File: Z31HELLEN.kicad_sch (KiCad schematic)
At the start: 2 parts, among them CON1 Z32 2024, CON2 Z32 2024

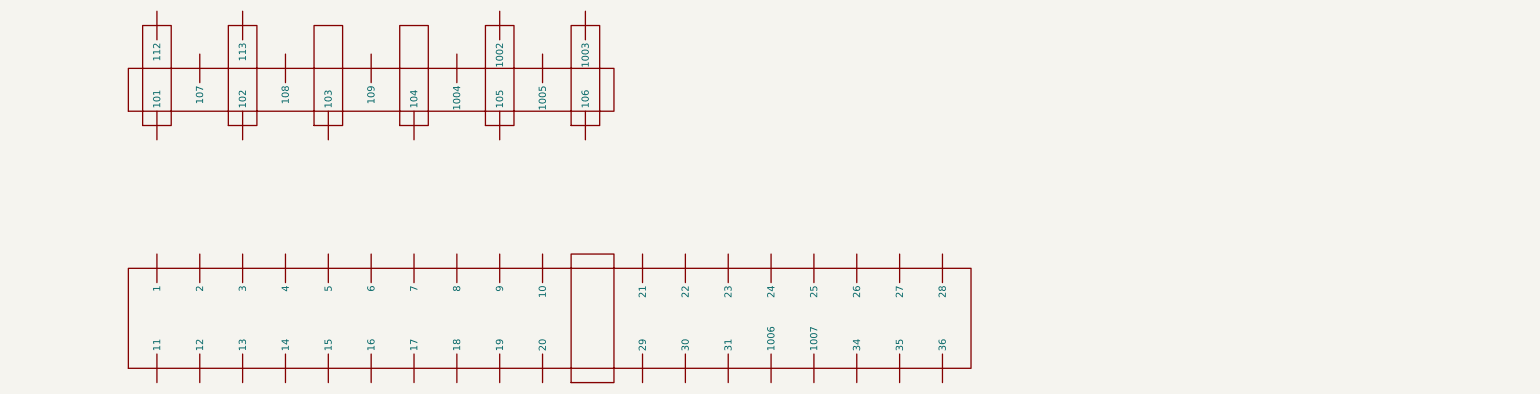
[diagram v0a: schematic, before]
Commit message: Add files via upload
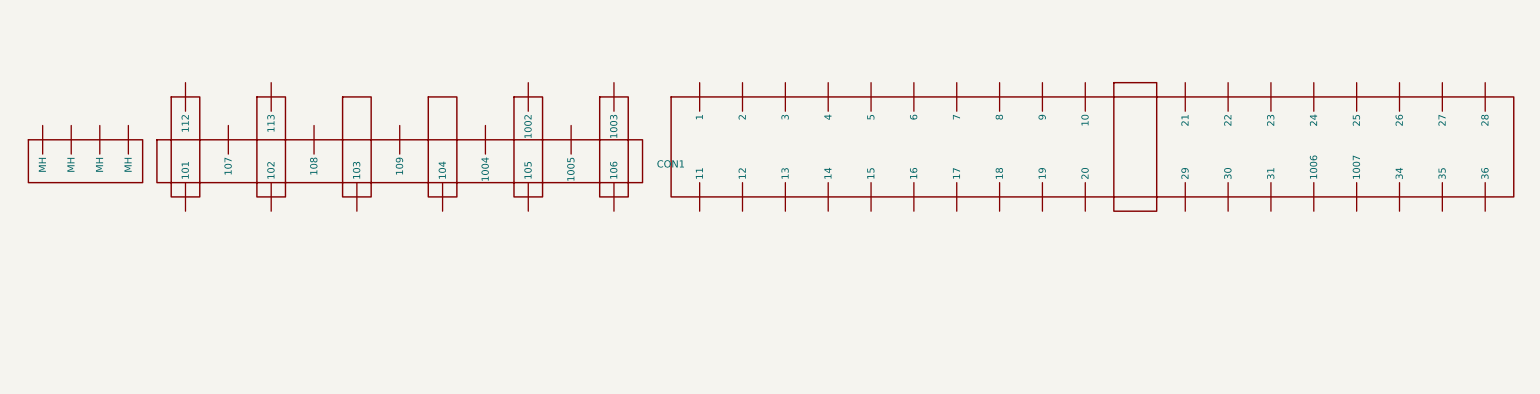
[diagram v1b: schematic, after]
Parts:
- removed CON1: Z32 2024, Main Conne-easyedapro:Z32 2024, symbol z31 15p:Z32 2024
- removed CON2: Z32 2024, Main Conne-easyedapro:Z32 2024, symbol 172023-1:Z32 2024
- added CON1: Z32 2024, symbol Z31HELLEN-altium-import:root_0_Z32 2024
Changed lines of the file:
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@@
 	(generator "eeschema")
 	(generator_version "8.0")
-	(paper "A4")
+	(paper "User" 274.32 99.06)
 	(symbol
-		(lib_id "z31 15p:Z32 2024")
-		(at 111.76 39.37 0)
+		(lib_id "Z31HELLEN-altium-import:root_0_Z32 2024")
+		(at 116.84 52.07 0)
 		(unit 1)
 		(exclude_from_sim no)
@@
 		(on_board yes)
 		(dnp no)
-		(fields_autoplaced yes)
 		(property "Reference" "CON1"
-			(at 265.43 24.13 0)
-			(effects
-				(font
-					(size 1.27 1.27)
-				)
-				(justify left bottom)
-				(hide yes)
+			(at 116.84 52.07 0)
+			(effects
+				(font
+					(size 1.27 1.27)
+				)
+				(justify left bottom)
 			)
 		)
 		(property "Value" "Z32 2024"
-			(at 265.43 26.162 0)
-			(effects
-				(font
-					(size 1.27 1.27)
-				)
-				(justify left bottom)
-				(hide yes)
-			)
-		)
-		(property "Footprint" "Main Conne-easyedapro:Z32 2024"
-			(at 111.76 39.37 0)
+			(at 116.84 52.07 0)
+			(effects
+				(font
+					(size 1.27 1.27)
+				)
+				(justify left bottom)
+				(hide yes)
+			)
+		)
+		(property "Footprint" ""
+			(at 116.84 52.07 0)
 			(effects
 				(font
@@
 		)
 		(property "Datasheet" ""
-			(at 111.76 39.37 0)
+			(at 116.84 52.07 0)
 			(effects
 				(font
@@
 		)
 		(property "Description" ""
-			(at 111.76 39.37 0)
-			(effects
-				(font
-					(size 1.27 1.27)
-				)
-				(hide yes)
-			)
+			(at 116.84 52.07 0)
+			(effects
+				(font
+					(size 1.27 1.27)
+				)
+				(hide yes)
+			)
+		)
+		(property "NAME" ""
+			(at 116.84 52.07 0)
+			(effects
+				(font
+					(size 1.27 1.27)
+				)
+				(justify left bottom)
+				(hide yes)
+			)
+		)
+		(property "SYMBOL" "Z32 2024"
+			(at 116.84 52.07 0)
+			(effects
+				(font
+					(size 1.27 1.27)
+				)
+				(justify left bottom)
+				(hide yes)
+			)
+		)
+		(property "DEVICE" "Z32 2024"
+			(at 116.84 52.07 0)
+			(effects
+				(font
+					(size 1.27 1.27)
+				)
+				(justify left bottom)
+				(hide yes)
+			)
+		)
+		(property "ADD INTO BOM" "yes"
+			(at 116.84 52.07 0)
+			(effects
+				(font
+					(size 1.27 1.27)
+				)
+				(justify left bottom)
+				(hide yes)
+			)
+		)
+		(property "CONVERT TO PCB" "yes"
+			(at 116.84 52.07 0)
+			(effects
+				(font
+					(size 1.27 1.27)
+				)
+				(justify left bottom)
+				(hide yes)
+			)
+		)
+		(property "MANUFACTURER" ""
+			(at 116.84 52.07 0)
+			(effects
+				(font
+					(size 1.27 1.27)
+				)
+				(justify left bottom)
+				(hide yes)
+			)
+		)
+		(property "MANUFACTURER PART" ""
+			(at 116.84 52.07 0)
+			(effects
+				(font
+					(size 1.27 1.27)
+				)
+				(justify left bottom)
+				(hide yes)
+			)
+		)
+		(property "SUPPLIER" ""
+			(at 116.84 52.07 0)
+			(effects
+				(font
+					(size 1.27 1.27)
+				)
+				(justify left bottom)
+				(hide yes)
+			)
+		)
+		(property "SUPPLIER PART" ""
+			(at 116.84 52.07 0)
+			(effects
+				(font
+					(size 1.27 1.27)
+				)
+				(justify left bottom)
+				(hide yes)
+			)
+		)
+		(property "_" "3"
+			(at 116.84 52.07 0)
+			(effects
+				(font
+					(size 1.27 1.27)
+				)
+				(justify left bottom)
+				(hide yes)
+			)
+		)
+		(property "DESCRIPTION" ""
+			(at 116.84 52.07 0)
+			(effects
+				(font
+					(size 1.27 1.27)
+				)
+				(justify left bottom)
+				(hide yes)
+			)
+		)
+		(pin "1008"
+		)
+		(pin "104"
+		)
+		(pin "106"
+		)
+		(pin "105"
+		)
+		(pin "103"
+		)
+		(pin "1007"
+		)
+		(pin "29"
+		)
+		(pin "30"
+		)
+		(pin "35"
+		)
+		(pin "28"
+		)
+		(pin "31"
+		)
+		(pin "27"
+		)
+		(pin "26"
+		)
+		(pin "3"
+		)
+		(pin "36"
+		)
+		(pin "1006"
+		)
+		(pin "107"
+		)
+		(pin "1005"
+		)
+		(pin "108"
+		)
+		(pin "1002"
+		)
+		(pin "1004"
+		)
+		(pin "112"
+		)
+		(pin "109"
+		)
+		(pin "1003"
+		)
+		(pin "101"
+		)
+		(pin "113"
 		)
 		(pin "102"
 		)
-		(pin "103"
-		)
-		(pin "1003"
-		)
-		(pin "101"
-		)
-		(pin "109"
-		)
-		(pin "105"
-		)
-		(pin "108"
-		)
-		(pin "112"
-		)
-		(pin "1004"
-		)
-		(pin "113"
-		)
-		(pin "107"
-		)
-		(pin "106"
-		)
-		(pin "1002"
-		)
-		(pin "104"
-		)
-		(pin "1005"
+		(pin "10010"
+		)
+		(pin "1009"
+		)
+		(pin "10011"
+		)
+		(pin "25"
+		)
+		(pin "16"
+		)
+		(pin "15"
+		)
+		(pin "23"
+		)
+		(pin "22"
+		)
+		(pin "20"
+		)
+		(pin "18"
+		)
+		(pin "17"
+		)
+		(pin "24"
+		)
+		(pin "21"
+		)
+		(pin "19"
+		)
+		(pin "34"
+		)
+		(pin "2"
+		)
+		(pin "1"
+		)
+		(pin "14"
+		)
+		(pin "12"
+		)
+		(pin "11"
+		)
+		(pin "9"
+		)
+		(pin "5"
+		)
+		(pin "10"
+		)
+		(pin "7"
+		)
+		(pin "6"
+		)
+		(pin "4"
+		)
+		(pin "13"
+		)
+		(pin "8"
 		)
 		(instances
 			(project ""
-				(path "/8bd93ac5-a5f9-4744-8cea-27f2f6693e74"
+				(path "/b506e640-3a9c-47d7-91fd-18e11bf19b9e"
 					(reference "CON1")
-					(unit 1)
-				)
-			)
-		)
-	)
-	(symbol
-		(lib_id "172023-1:Z32 2024")
-		(at 20.32 82.55 0)
-		(unit 1)
-		(exclude_from_sim no)
-		(in_bom yes)
-		(on_board yes)
-		(dnp no)
-		(fields_autoplaced yes)
-		(property "Reference" "CON2"
-			(at 173.99 67.31 0)
-			(effects
-				(font
-					(size 1.27 1.27)
-				)
-				(justify left bottom)
-				(hide yes)
-			)
-		)
-		(property "Value" "Z32 2024"
-			(at 173.99 69.342 0)
-			(effects
-				(font
-					(size 1.27 1.27)
-				)
-				(justify left bottom)
-				(hide yes)
-			)
-		)
-		(property "Footprint" "Main Conne-easyedapro:Z32 2024"
-			(at 20.32 82.55 0)
-			(effects
-				(font
-					(size 1.27 1.27)
-				)
-				(hide yes)
-			)
-		)
-		(property "Datasheet" ""
-			(at 20.32 82.55 0)
-			(effects
-				(font
-					(size 1.27 1.27)
-				)
-				(hide yes)
-			)
-		)
-		(property "Description" ""
-			(at 20.32 82.55 0)
-			(effects
-				(font
-					(size 1.27 1.27)
-				)
-				(hide yes)
-			)
-		)
-		(pin "26"
-		)
-		(pin "28"
-		)
-		(pin "16"
-		)
-		(pin "29"
-		)
-		(pin "10"
-		)
-		(pin "14"
-		)
-		(pin "1006"
-		)
-		(pin "35"
-		)
-		(pin "27"
-		)
-		(pin "31"
-		)
-		(pin "34"
-		)
-		(pin "36"
-		)
-		(pin "24"
-		)
-		(pin "1007"
-		)
-		(pin "12"
-		)
-		(pin "30"
-		)
-		(pin "17"
-		)
-		(pin "18"
-		)
-		(pin "3"
-		)
-		(pin "4"
-		)
-		(pin "22"
-		)
-		(pin "2"
-		)
-		(pin "1"
-		)
-		(pin "11"
-		)
-		(pin "15"
-		)
-		(pin "19"
-		)
-		(pin "20"
-		)
-		(pin "21"
-		)
-		(pin "13"
-		)
-		(pin "23"
-		)
-		(pin "25"
-		)
-		(pin "9"
-		)
-		(pin "8"
-		)
-		(pin "6"
-		)
-		(pin "5"
-		)
-		(pin "7"
-		)
-		(instances
-			(project ""
-				(path "/8bd93ac5-a5f9-4744-8cea-27f2f6693e74"
-					(reference "CON2")
 					(unit 1)
 				)
@@
 	(sheet_instances
 		(path "/"
-			(page "1")
+			(page "#")
 		)
 	)

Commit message: Add files via upload
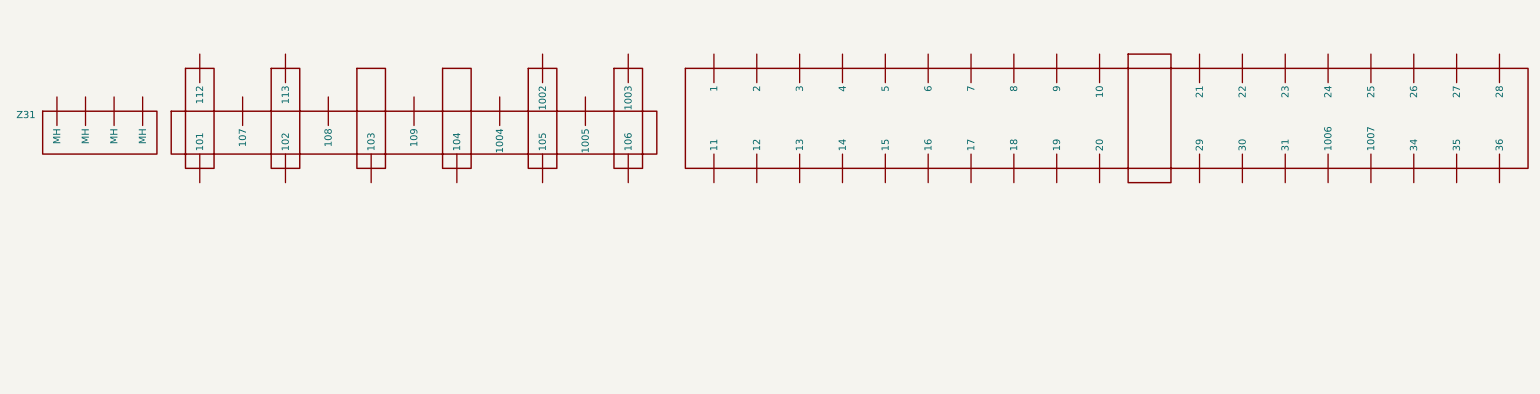
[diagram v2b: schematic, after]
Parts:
- removed CON1: Z32 2024, symbol Z31HELLEN-altium-import:root_0_Z32 2024
- added Z31: ~, Z31:Z31 15 + 36, symbol Z31HELLEN-altium-import:root_0_Z32 2024
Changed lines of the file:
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@@
 	(symbol
 		(lib_id "Z31HELLEN-altium-import:root_0_Z32 2024")
-		(at 116.84 52.07 0)
+		(at 119.38 46.99 0)
 		(unit 1)
 		(exclude_from_sim no)
@@
 		(on_board yes)
 		(dnp no)
-		(property "Reference" "CON1"
-			(at 116.84 52.07 0)
+		(fields_autoplaced yes)
+		(property "Reference" "Z31"
+			(at 6.35 42.5449 0)
 			(effects
 				(font
 					(size 1.27 1.27)
 				)
-				(justify left bottom)
+				(justify right)
 			)
 		)
-		(property "Value" "Z32 2024"
-			(at 116.84 52.07 0)
+		(property "Value" "~"
+			(at 6.35 44.45 0)
 			(effects
 				(font
 					(size 1.27 1.27)
 				)
-				(justify left bottom)
-				(hide yes)
+				(justify right)
 			)
 		)
-		(property "Footprint" ""
-			(at 116.84 52.07 0)
+		(property "Footprint" "Z31:Z31 15 + 36"
+			(at 119.38 46.99 0)
 			(effects
 				(font
@@
 		)
 		(property "Datasheet" ""
-			(at 116.84 52.07 0)
+			(at 119.38 46.99 0)
 			(effects
 				(font
@@
 		)
 		(property "Description" ""
-			(at 116.84 52.07 0)
+			(at 119.38 46.99 0)
 			(effects
 				(font
@@
 			)
 		)
-		(property "NAME" ""
-			(at 116.84 52.07 0)
-			(effects
-				(font
-					(size 1.27 1.27)
-				)
-				(justify left bottom)
-				(hide yes)
-			)
+		(pin "1009"
 		)
-		(property "SYMBOL" "Z32 2024"
-			(at 116.84 52.07 0)
-			(effects
-				(font
-					(size 1.27 1.27)
-				)
-				(justify left bottom)
-				(hide yes)
-			)
+		(pin "2"
 		)
-		(property "DEVICE" "Z32 2024"
-			(at 116.84 52.07 0)
-			(effects
-				(font
-					(size 1.27 1.27)
-				)
-				(justify left bottom)
-				(hide yes)
-			)
+		(pin "21"
 		)
-		(property "ADD INTO BOM" "yes"
-			(at 116.84 52.07 0)
-			(effects
-				(font
-					(size 1.27 1.27)
-				)
-				(justify left bottom)
-				(hide yes)
-			)
+		(pin "24"
 		)
-		(property "CONVERT TO PCB" "yes"
-			(at 116.84 52.07 0)
-			(effects
-				(font
-					(size 1.27 1.27)
-				)
-				(justify left bottom)
-				(hide yes)
-			)
+		(pin "27"
 		)
-		(property "MANUFACTURER" ""
-			(at 116.84 52.07 0)
-			(effects
-				(font
-					(size 1.27 1.27)
-				)
-				(justify left bottom)
-				(hide yes)
-			)
+		(pin "112"
 		)
-		(property "MANUFACTURER PART" ""
-			(at 116.84 52.07 0)
-			(effects
-				(font
-					(size 1.27 1.27)
-				)
-				(justify left bottom)
-				(hide yes)
-			)
+		(pin "28"
 		)
-		(property "SUPPLIER" ""
-			(at 116.84 52.07 0)
-			(effects
-				(font
-					(size 1.27 1.27)
-				)
-				(justify left bottom)
-				(hide yes)
-			)
+		(pin "102"
 		)
-		(property "SUPPLIER PART" ""
-			(at 116.84 52.07 0)
-			(effects
-				(font
-					(size 1.27 1.27)
-				)
-				(justify left bottom)
-				(hide yes)
-			)
+		(pin "23"
 		)
-		(property "_" "3"
-			(at 116.84 52.07 0)
-			(effects
-				(font
-					(size 1.27 1.27)
-				)
-				(justify left bottom)
-				(hide yes)
-			)
+		(pin "26"
 		)
-		(property "DESCRIPTION" ""
-			(at 116.84 52.07 0)
-			(effects
-				(font
-					(size 1.27 1.27)
-				)
-				(justify left bottom)
-				(hide yes)
-			)
+		(pin "14"
+		)
+		(pin "1004"
+		)
+		(pin "107"
+		)
+		(pin "15"
+		)
+		(pin "19"
+		)
+		(pin "13"
+		)
+		(pin "25"
+		)
+		(pin "106"
+		)
+		(pin "1006"
+		)
+		(pin "108"
+		)
+		(pin "109"
+		)
+		(pin "1005"
+		)
+		(pin "16"
+		)
+		(pin "103"
+		)
+		(pin "104"
+		)
+		(pin "17"
+		)
+		(pin "20"
+		)
+		(pin "10"
+		)
+		(pin "1003"
+		)
+		(pin "22"
+		)
+		(pin "29"
+		)
+		(pin "3"
+		)
+		(pin "10010"
+		)
+		(pin "113"
+		)
+		(pin "1"
+		)
+		(pin "10011"
 		)
 		(pin "1008"
 		)
-		(pin "104"
+		(pin "101"
 		)
-		(pin "106"
+		(pin "11"
+		)
+		(pin "12"
 		)
 		(pin "105"
 		)
-		(pin "103"
+		(pin "30"
+		)
+		(pin "18"
+		)
+		(pin "1002"
 		)
 		(pin "1007"
 		)
-		(pin "29"
-		)
-		(pin "30"
+		(pin "34"
 		)
 		(pin "35"
 		)
-		(pin "28"
+		(pin "9"
+		)
+		(pin "4"
+		)
+		(pin "8"
+		)
+		(pin "6"
+		)
+		(pin "5"
+		)
+		(pin "36"
 		)
 		(pin "31"
 		)
-		(pin "27"
-		)
-		(pin "26"
-		)
-		(pin "3"
-		)
-		(pin "36"
-		)
-		(pin "1006"
-		)
-		(pin "107"
-		)
-		(pin "1005"
-		)
-		(pin "108"
-		)
-		(pin "1002"
-		)
-		(pin "1004"
-		)
-		(pin "112"
-		)
-		(pin "109"
-		)
-		(pin "1003"
-		)
-		(pin "101"
-		)
-		(pin "113"
-		)
-		(pin "102"
-		)
-		(pin "10010"
-		)
-		(pin "1009"
-		)
-		(pin "10011"
-		)
-		(pin "25"
-		)
-		(pin "16"
-		)
-		(pin "15"
-		)
-		(pin "23"
-		)
-		(pin "22"
-		)
-		(pin "20"
-		)
-		(pin "18"
-		)
-		(pin "17"
-		)
-		(pin "24"
-		)
-		(pin "21"
-		)
-		(pin "19"
-		)
-		(pin "34"
-		)
-		(pin "2"
-		)
-		(pin "1"
-		)
-		(pin "14"
-		)
-		(pin "12"
-		)
-		(pin "11"
-		)
-		(pin "9"
-		)
-		(pin "5"
-		)
-		(pin "10"
-		)
 		(pin "7"
-		)
-		(pin "6"
-		)
-		(pin "4"
-		)
-		(pin "13"
-		)
-		(pin "8"
 		)
 		(instances
 			(project ""
 				(path "/b506e640-3a9c-47d7-91fd-18e11bf19b9e"
-					(reference "CON1")
+					(reference "Z31")
 					(unit 1)
 				)
